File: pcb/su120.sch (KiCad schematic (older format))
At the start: 142 parts, among them J1 MJ-4PP-9, J2 Conn_01x03, J3 Conn_01x08, J4 Conn_01x08, J5 Conn_01x03, J6 MJ-4PP-9, SW1 SW_Push, SW10 SW_Push, SW11 SW_Push, SW12 SW_Push, SW13 SW_Push, SW14 SW_Push, SW15 SW_Push, SW16 SW_Push, SW17 SW_Push, SW18 SW_Push, SW19 Rotary_Encoder_Switch, SW2 SW_Push, SW20 Rotary_Encoder_Switch, SW21 SW_Push, SW3 SW_Push, SW4 SW_Push, SW5 SW_Push, SW6 SW_Push, SW7 SW_Push, SW8 SW_Push, SW9 SW_Push, U1 ProMicro

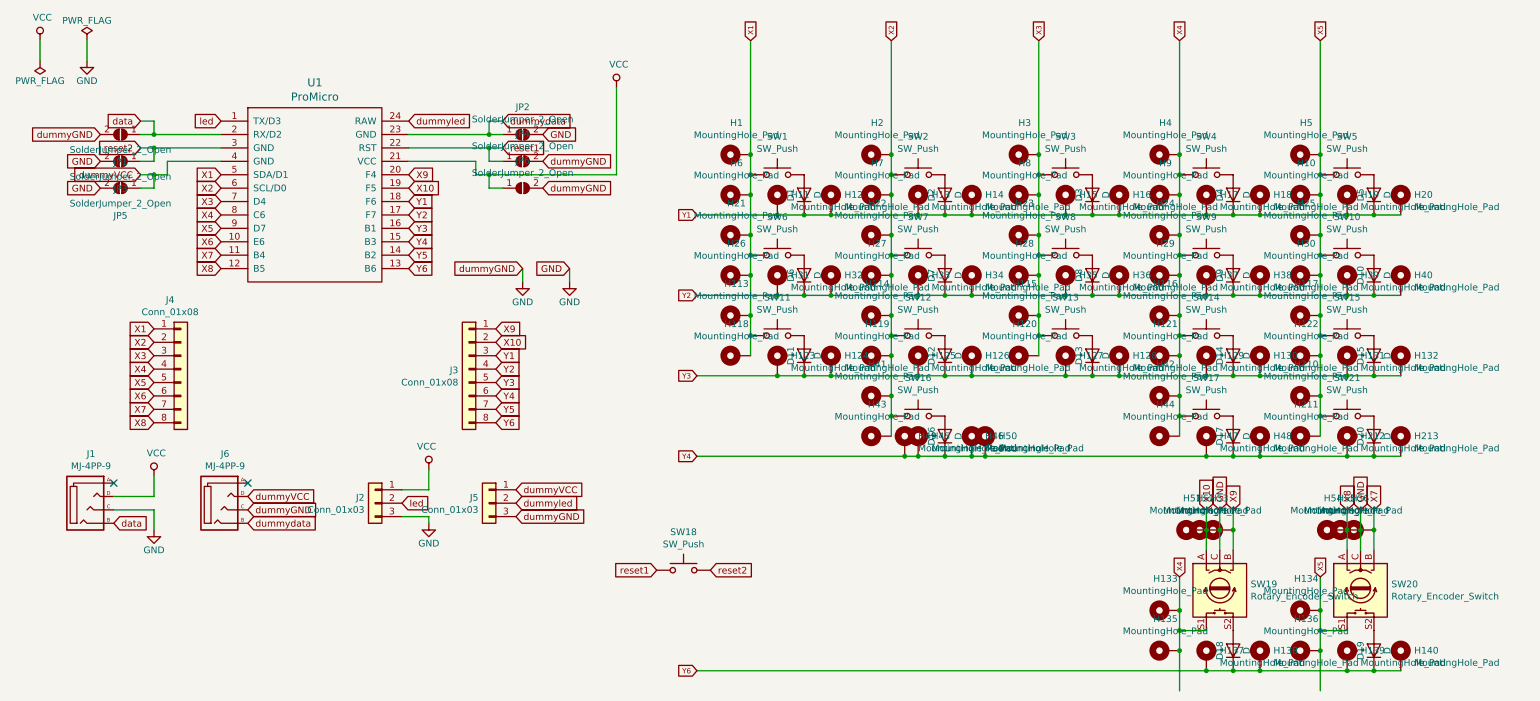
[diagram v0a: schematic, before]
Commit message: Rev.8
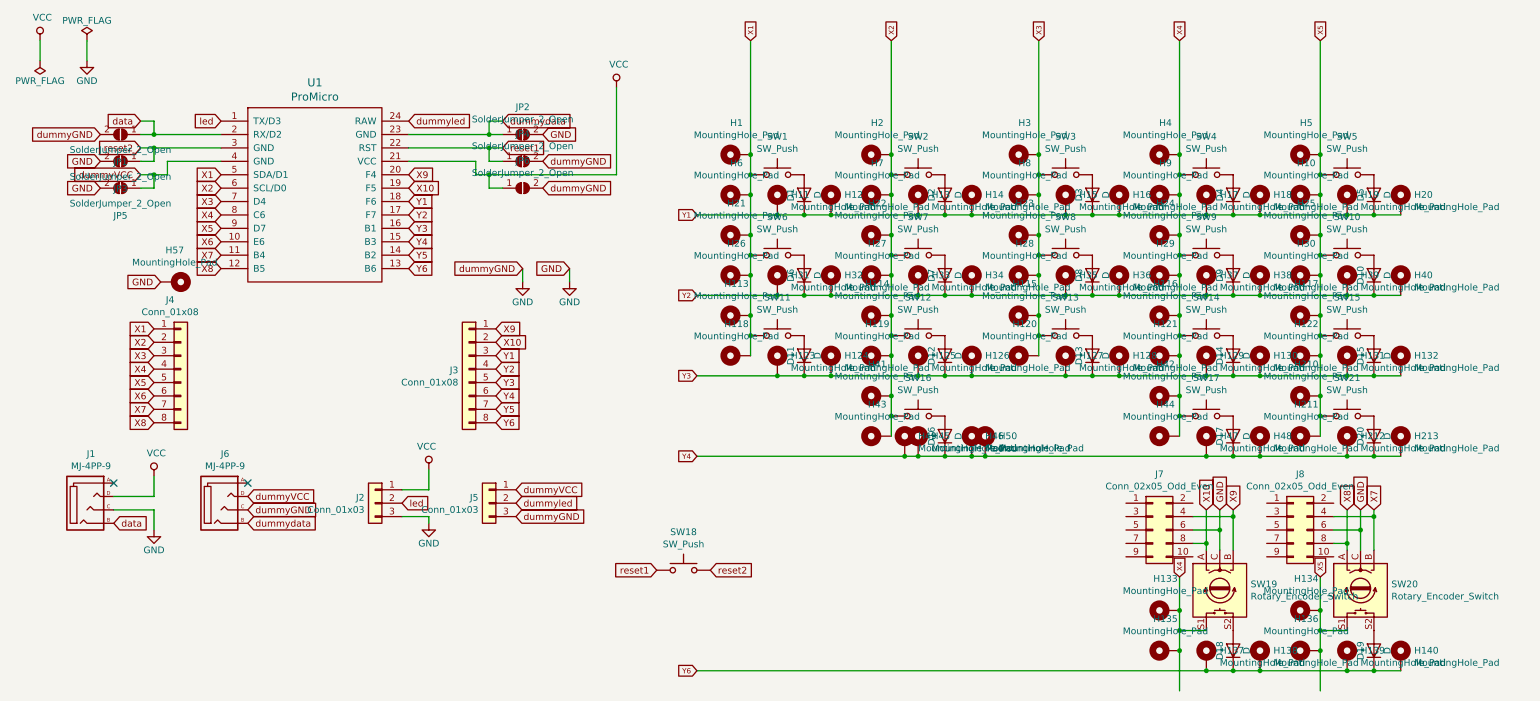
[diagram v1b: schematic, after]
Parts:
- removed H51, H52, H53, H54, H55, H56: MountingHole_Pad, #footprint:1pin_conn, symbol Mechanical:MountingHole_Pad
- added H57: MountingHole_Pad, #footprint:1pin_conn, symbol Mechanical:MountingHole_Pad
- added J7, J8: Conn_02x05_Odd_Even, #footprint:IDC-Header_2x05_P2.54mm_Vertical, symbol Connector_Generic:Conn_02x05_Odd_Even
- D1, D10, D11, D12, D13, D14, D15, D16, D17, D18, D19, D2, D20, D3, D4, D5, D6, D7, D8, D9: footprint #footprint:diode_TH_SMD -> #footprint:diode_TH_SMD_rev2
- SW21: footprint #footprint:CherryMX_Choc_Hotswap_rev4 -> #footprint:CherryMX_MidHeight_Choc_Hotswap_rev5
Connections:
- net GND: now also H57.1, J7.6 (Pin_6), J8.6 (Pin_6)
- net X10: now also J7.8 (Pin_8)
- net X7: now also J8.4 (Pin_4)
- net X8: now also J8.8 (Pin_8)
- net X9: now also J7.4 (Pin_4)
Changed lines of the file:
@@
 Title "SU120 Yakitori Keyboard"
 Date ""
-Rev "7"
+Rev "8"
 Comp "@e3w2q"
 Comment1 ""
@@
 F 0 "D1" H 6400 2050 50  0000 C CNN
 F 1 "D" H 6400 1850 50  0000 C CNN
-F 2 "#footprint:diode_TH_SMD" H 6400 1950 50  0001 C CNN
+F 2 "#footprint:diode_TH_SMD_rev2" H 6400 1950 50  0001 C CNN
 F 3 "" H 6400 1950 50  0001 C CNN
 	1    6400 1950
@@
 F 0 "D2" H 7450 2050 50  0000 C CNN
 F 1 "D" H 7450 1850 50  0000 C CNN
-F 2 "#footprint:diode_TH_SMD" H 7450 1950 50  0001 C CNN
+F 2 "#footprint:diode_TH_SMD_rev2" H 7450 1950 50  0001 C CNN
 F 3 "" H 7450 1950 50  0001 C CNN
 	1    7450 1950
@@
 F 0 "D3" H 8550 2050 50  0000 C CNN
 F 1 "D" H 8550 1850 50  0000 C CNN
-F 2 "#footprint:diode_TH_SMD" H 8550 1950 50  0001 C CNN
+F 2 "#footprint:diode_TH_SMD_rev2" H 8550 1950 50  0001 C CNN
 F 3 "" H 8550 1950 50  0001 C CNN
 	1    8550 1950
@@
 F 0 "D4" H 9600 2050 50  0000 C CNN
 F 1 "D" H 9600 1850 50  0000 C CNN
-F 2 "#footprint:diode_TH_SMD" H 9600 1950 50  0001 C CNN
+F 2 "#footprint:diode_TH_SMD_rev2" H 9600 1950 50  0001 C CNN
 F 3 "" H 9600 1950 50  0001 C CNN
 	1    9600 1950
@@
 F 0 "D6" H 6400 2650 50  0000 C CNN
 F 1 "D" H 6400 2450 50  0000 C CNN
-F 2 "#footprint:diode_TH_SMD" H 6400 2550 50  0001 C CNN
+F 2 "#footprint:diode_TH_SMD_rev2" H 6400 2550 50  0001 C CNN
 F 3 "" H 6400 2550 50  0001 C CNN
 	1    6400 2550
@@
 F 0 "D7" H 7450 2650 50  0000 C CNN
 F 1 "D" H 7450 2450 50  0000 C CNN
-F 2 "#footprint:diode_TH_SMD" H 7450 2550 50  0001 C CNN
+F 2 "#footprint:diode_TH_SMD_rev2" H 7450 2550 50  0001 C CNN
 F 3 "" H 7450 2550 50  0001 C CNN
 	1    7450 2550
@@
 F 0 "D8" H 8550 2650 50  0000 C CNN
 F 1 "D" H 8550 2450 50  0000 C CNN
-F 2 "#footprint:diode_TH_SMD" H 8550 2550 50  0001 C CNN
+F 2 "#footprint:diode_TH_SMD_rev2" H 8550 2550 50  0001 C CNN
 F 3 "" H 8550 2550 50  0001 C CNN
 	1    8550 2550
@@
 F 0 "D9" H 9600 2650 50  0000 C CNN
 F 1 "D" H 9600 2450 50  0000 C CNN
-F 2 "#footprint:diode_TH_SMD" H 9600 2550 50  0001 C CNN
+F 2 "#footprint:diode_TH_SMD_rev2" H 9600 2550 50  0001 C CNN
 F 3 "" H 9600 2550 50  0001 C CNN
 	1    9600 2550
@@
 F 0 "D5" H 10650 2050 50  0000 C CNN
 F 1 "D" H 10650 1850 50  0000 C CNN
-F 2 "#footprint:diode_TH_SMD" H 10650 1950 50  0001 C CNN
+F 2 "#footprint:diode_TH_SMD_rev2" H 10650 1950 50  0001 C CNN
 F 3 "" H 10650 1950 50  0001 C CNN
 	1    10650 1950
@@
 F 0 "D10" H 10650 2650 50  0000 C CNN
 F 1 "D" H 10650 2450 50  0000 C CNN
-F 2 "#footprint:diode_TH_SMD" H 10650 2550 50  0001 C CNN
+F 2 "#footprint:diode_TH_SMD_rev2" H 10650 2550 50  0001 C CNN
 F 3 "" H 10650 2550 50  0001 C CNN
 	1    10650 2550
@@
 F 0 "D16" H 7450 3850 50  0000 C CNN
 F 1 "D" H 7450 3650 50  0000 C CNN
-F 2 "#footprint:diode_TH_SMD" H 7450 3750 50  0001 C CNN
+F 2 "#footprint:diode_TH_SMD_rev2" H 7450 3750 50  0001 C CNN
 F 3 "" H 7450 3750 50  0001 C CNN
 	1    7450 3750
@@
 F 0 "D17" H 9600 3850 50  0000 C CNN
 F 1 "D" H 9600 3650 50  0000 C CNN
-F 2 "#footprint:diode_TH_SMD" H 9600 3750 50  0001 C CNN
+F 2 "#footprint:diode_TH_SMD_rev2" H 9600 3750 50  0001 C CNN
 F 3 "" H 9600 3750 50  0001 C CNN
 	1    9600 3750
@@
 F 0 "D11" H 6400 3250 50  0000 C CNN
 F 1 "D" H 6400 3050 50  0000 C CNN
-F 2 "#footprint:diode_TH_SMD" H 6400 3150 50  0001 C CNN
+F 2 "#footprint:diode_TH_SMD_rev2" H 6400 3150 50  0001 C CNN
 F 3 "" H 6400 3150 50  0001 C CNN
 	1    6400 3150
@@
 F 0 "D12" H 7450 3250 50  0000 C CNN
 F 1 "D" H 7450 3050 50  0000 C CNN
-F 2 "#footprint:diode_TH_SMD" H 7450 3150 50  0001 C CNN
+F 2 "#footprint:diode_TH_SMD_rev2" H 7450 3150 50  0001 C CNN
 F 3 "" H 7450 3150 50  0001 C CNN
 	1    7450 3150
@@
 F 0 "D13" H 8550 3250 50  0000 C CNN
 F 1 "D" H 8550 3050 50  0000 C CNN
-F 2 "#footprint:diode_TH_SMD" H 8550 3150 50  0001 C CNN
+F 2 "#footprint:diode_TH_SMD_rev2" H 8550 3150 50  0001 C CNN
 F 3 "" H 8550 3150 50  0001 C CNN
 	1    8550 3150
@@
 F 0 "D14" H 9600 3250 50  0000 C CNN
 F 1 "D" H 9600 3050 50  0000 C CNN
-F 2 "#footprint:diode_TH_SMD" H 9600 3150 50  0001 C CNN
+F 2 "#footprint:diode_TH_SMD_rev2" H 9600 3150 50  0001 C CNN
 F 3 "" H 9600 3150 50  0001 C CNN
 	1    9600 3150
@@
 F 0 "D15" H 10650 3250 50  0000 C CNN
 F 1 "D" H 10650 3050 50  0000 C CNN
-F 2 "#footprint:diode_TH_SMD" H 10650 3150 50  0001 C CNN
+F 2 "#footprint:diode_TH_SMD_rev2" H 10650 3150 50  0001 C CNN
 F 3 "" H 10650 3150 50  0001 C CNN
 	1    10650 3150
@@
 F 0 "D18" H 9600 5450 50  0000 C CNN
 F 1 "D" H 9600 5250 50  0000 C CNN
-F 2 "#footprint:diode_TH_SMD" H 9600 5350 50  0001 C CNN
+F 2 "#footprint:diode_TH_SMD_rev2" H 9600 5350 50  0001 C CNN
 F 3 "" H 9600 5350 50  0001 C CNN
 	1    9600 5350
@@
 F 0 "D19" H 10650 5450 50  0000 C CNN
 F 1 "D" H 10650 5250 50  0000 C CNN
-F 2 "#footprint:diode_TH_SMD" H 10650 5350 50  0001 C CNN
+F 2 "#footprint:diode_TH_SMD_rev2" H 10650 5350 50  0001 C CNN
 F 3 "" H 10650 5350 50  0001 C CNN
 	1    10650 5350
@@
 F 0 "D20" H 10650 3850 50  0000 C CNN
 F 1 "D" H 10650 3650 50  0000 C CNN
-F 2 "#footprint:diode_TH_SMD" H 10650 3750 50  0001 C CNN
+F 2 "#footprint:diode_TH_SMD_rev2" H 10650 3750 50  0001 C CNN
 F 3 "" H 10650 3750 50  0001 C CNN
 	1    10650 3750
@@
 F 0 "SW21" H 10450 3885 50  0000 C CNN
 F 1 "SW_Push" H 10450 3794 50  0000 C CNN
-F 2 "#footprint:CherryMX_Choc_Hotswap_rev4" H 10450 3800 50  0001 C CNN
+F 2 "#footprint:CherryMX_MidHeight_Choc_Hotswap_rev5" H 10450 3800 50  0001 C CNN
 F 3 "" H 10450 3800 50  0001 C CNN
 	1    10450 3600
@@
 X10
 $Comp
-L Mechanical:MountingHole_Pad H51
-U 1 1 5D672636
-P 9300 4450
-F 0 "H51" V 9537 4455 50  0000 C CNN
-F 1 "MountingHole_Pad" V 9446 4455 50  0000 C CNN
-F 2 "#footprint:1pin_conn" H 9300 4450 50  0001 C CNN
-F 3 "~" H 9300 4450 50  0001 C CNN
-	1    9300 4450
-	0    -1   -1   0
-$EndComp
-$Comp
-L Mechanical:MountingHole_Pad H52
-U 1 1 5D67276C
-P 9400 4450
-F 0 "H52" V 9637 4455 50  0000 C CNN
-F 1 "MountingHole_Pad" V 9546 4455 50  0000 C CNN
-F 2 "#footprint:1pin_conn" H 9400 4450 50  0001 C CNN
-F 3 "~" H 9400 4450 50  0001 C CNN
-	1    9400 4450
-	0    -1   -1   0
-$EndComp
-$Comp
-L Mechanical:MountingHole_Pad H53
-U 1 1 5D672890
-P 9500 4450
-F 0 "H53" V 9737 4455 50  0000 C CNN
-F 1 "MountingHole_Pad" V 9646 4455 50  0000 C CNN
-F 2 "#footprint:1pin_conn" H 9500 4450 50  0001 C CNN
-F 3 "~" H 9500 4450 50  0001 C CNN
-	1    9500 4450
-	0    -1   -1   0
-$EndComp
-$Comp
-L Mechanical:MountingHole_Pad H54
-U 1 1 5D672A90
-P 10350 4450
-F 0 "H54" V 10587 4455 50  0000 C CNN
-F 1 "MountingHole_Pad" V 10496 4455 50  0000 C CNN
-F 2 "#footprint:1pin_conn" H 10350 4450 50  0001 C CNN
-F 3 "~" H 10350 4450 50  0001 C CNN
-	1    10350 4450
-	0    -1   -1   0
-$EndComp
-$Comp
-L Mechanical:MountingHole_Pad H55
-U 1 1 5D672A96
-P 10450 4450
-F 0 "H55" V 10687 4455 50  0000 C CNN
-F 1 "MountingHole_Pad" V 10596 4455 50  0000 C CNN
-F 2 "#footprint:1pin_conn" H 10450 4450 50  0001 C CNN
-F 3 "~" H 10450 4450 50  0001 C CNN
-	1    10450 4450
-	0    -1   -1   0
-$EndComp
-$Comp
-L Mechanical:MountingHole_Pad H56
-U 1 1 5D672A9C
-P 10550 4450
-F 0 "H56" V 10787 4455 50  0000 C CNN
-F 1 "MountingHole_Pad" V 10696 4455 50  0000 C CNN
-F 2 "#footprint:1pin_conn" H 10550 4450 50  0001 C CNN
-F 3 "~" H 10550 4450 50  0001 C CNN
-	1    10550 4450
-	0    -1   -1   0
-$EndComp
-Wire Wire Line
-	9400 4300 9400 4450
-Connection ~ 9400 4450
-Wire Wire Line
-	9400 4450 9400 4600
+L Mechanical:MountingHole_Pad H57
+U 1 1 5E0F561B
+P 1700 2600
+F 0 "H57" V 1937 2605 50  0000 C CNN
+F 1 "MountingHole_Pad" V 1846 2605 50  0000 C CNN
+F 2 "#footprint:1pin_conn" H 1700 2600 50  0001 C CNN
+F 3 "~" H 1700 2600 50  0001 C CNN
+	1    1700 2600
+	0    1    -1   0
+$EndComp
+Text GLabel 1600 2600 0    50   Input ~ 0
+GND
+$Comp
+L Connector_Generic:Conn_02x05_Odd_Even J8
+U 1 1 5E124F08
+P 10050 4450
+F 0 "J8" H 10100 4867 50  0000 C CNN
+F 1 "Conn_02x05_Odd_Even" H 10100 4776 50  0000 C CNN
+F 2 "#footprint:IDC-Header_2x05_P2.54mm_Vertical" H 10050 4450 50  0001 C CNN
+F 3 "~" H 10050 4450 50  0001 C CNN
+	1    10050 4450
+	1    0    0    -1
+$EndComp
+$Comp
+L Connector_Generic:Conn_02x05_Odd_Even J7
+U 1 1 5E113B23
+P 9000 4450
+F 0 "J7" H 9050 4867 50  0000 C CNN
+F 1 "Conn_02x05_Odd_Even" H 9050 4776 50  0000 C CNN
+F 2 "#footprint:IDC-Header_2x05_P2.54mm_Vertical" H 9000 4450 50  0001 C CNN
+F 3 "~" H 9000 4450 50  0001 C CNN
+	1    9000 4450
+	1    0    0    -1
+$EndComp
+Wire Wire Line
+	9400 4300 9400 4550
 Wire Wire Line
 	9500 4300 9500 4450
+Wire Wire Line
+	9600 4300 9600 4350
+Wire Wire Line
+	10450 4300 10450 4550
+Wire Wire Line
+	10550 4300 10550 4450
+Wire Wire Line
+	10650 4300 10650 4350
+Wire Wire Line
+	9300 4350 9600 4350
+Connection ~ 9600 4350
+Wire Wire Line
+	9600 4350 9600 4600
+Wire Wire Line
+	9300 4450 9500 4450
 Connection ~ 9500 4450
 Wire Wire Line
 	9500 4450 9500 4600
 Wire Wire Line
-	9600 4300 9600 4450
-Connection ~ 9600 4450
-Wire Wire Line
-	9600 4450 9600 4600
-Wire Wire Line
-	10450 4300 10450 4450
-Connection ~ 10450 4450
-Wire Wire Line
-	10450 4450 10450 4600
-Wire Wire Line
-	10550 4300 10550 4450
+	9300 4550 9400 4550
+Connection ~ 9400 4550
+Wire Wire Line
+	9400 4550 9400 4600
+Wire Wire Line
+	10350 4350 10650 4350
+Connection ~ 10650 4350
+Wire Wire Line
+	10650 4350 10650 4600
+Wire Wire Line
+	10350 4450 10550 4450
 Connection ~ 10550 4450
 Wire Wire Line
 	10550 4450 10550 4600
 Wire Wire Line
-	10650 4300 10650 4450
-Connection ~ 10650 4450
-Wire Wire Line
-	10650 4450 10650 4600
+	10350 4550 10450 4550
+Connection ~ 10450 4550
+Wire Wire Line
+	10450 4550 10450 4600
 $EndSCHEMATC
